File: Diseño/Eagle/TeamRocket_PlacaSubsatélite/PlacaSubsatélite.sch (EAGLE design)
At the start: 8 parts, among them IC2 7806DT

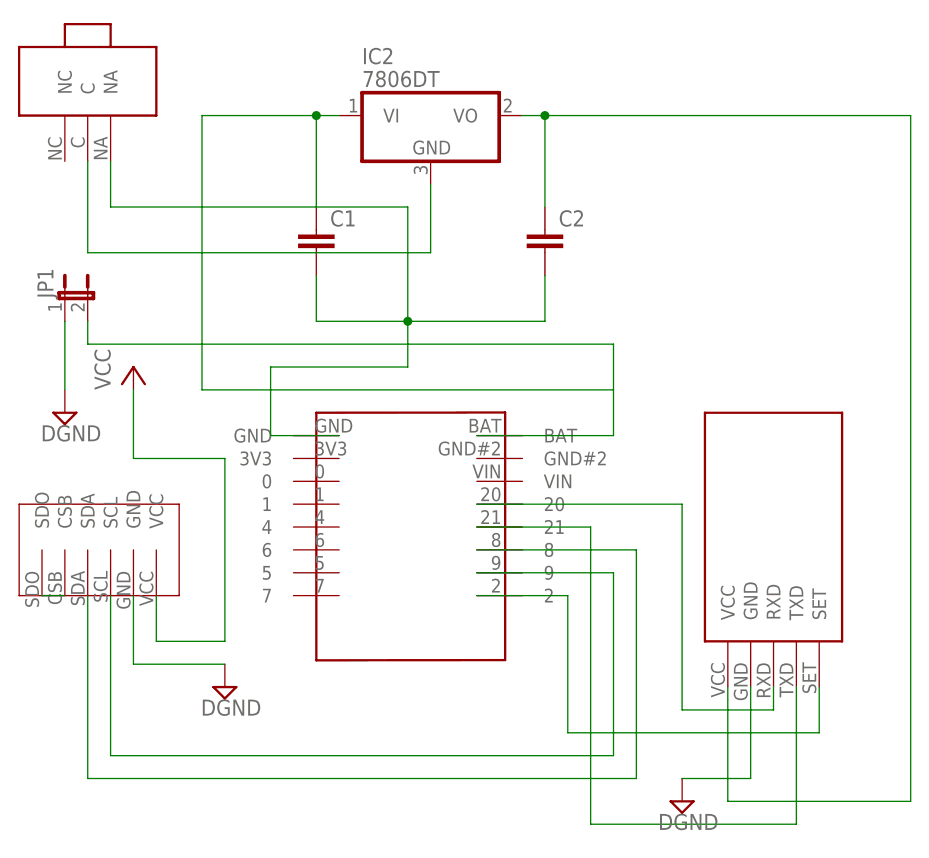
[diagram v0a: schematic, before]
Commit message: Update
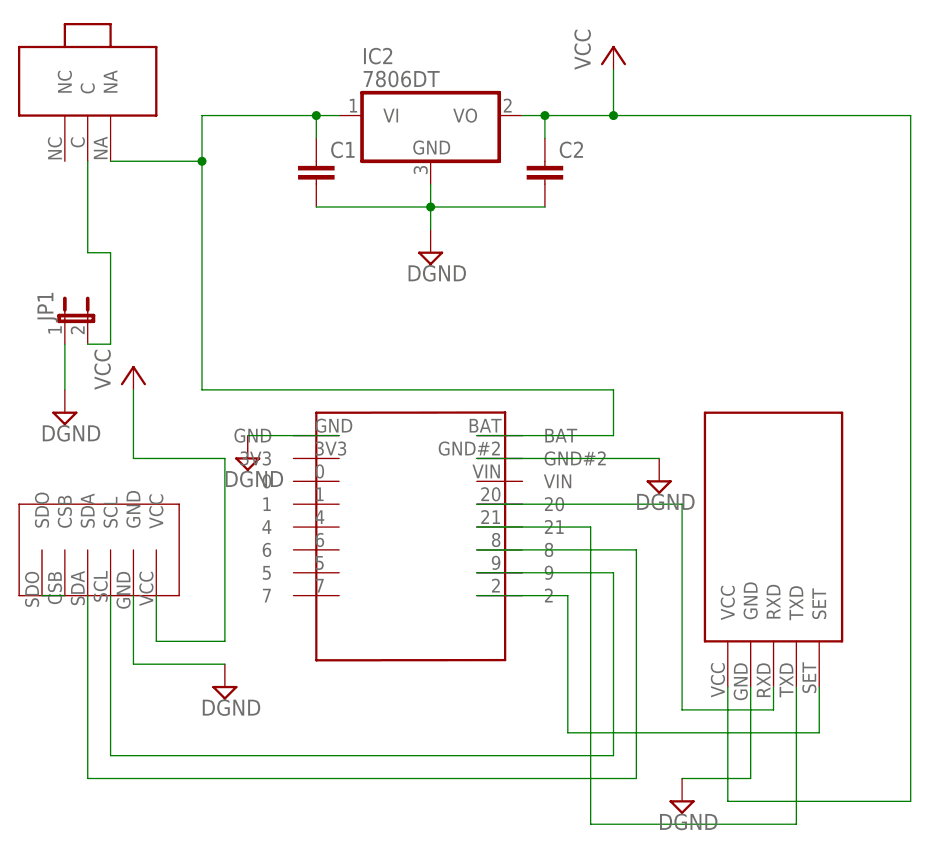
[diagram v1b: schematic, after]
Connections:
- removed net N$10: C2.1, IC2.VO, U$2.VCC
- removed net N$12: C1.2, C2.2, U$3.GND, U$4.NA
- net DGND: now also C1.2, C2.2, IC2.GND, U$3.GND, U$3.GND#2
- net N$1: now also U$4.NA; no longer JP1.2
- net N$2: now also JP1.2; no longer IC2.GND
- net VCC: now also C2.1, IC2.VO, U$2.VCC
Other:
- moved on the sheet: C1, C2, JP1
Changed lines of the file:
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@@
 <part name="SUPPLY3" library="supply2" library_urn="urn:adsk.eagle:library:372" deviceset="DGND" device=""/>
 <part name="U$4" library="switch" deviceset="SWITCH" device=""/>
+<part name="P+2" library="supply1" library_urn="urn:adsk.eagle:library:371" deviceset="VCC" device=""/>
+<part name="SUPPLY4" library="supply2" library_urn="urn:adsk.eagle:library:372" deviceset="DGND" device=""/>
+<part name="SUPPLY5" library="supply2" library_urn="urn:adsk.eagle:library:372" deviceset="DGND" device=""/>
+<part name="SUPPLY6" library="supply2" library_urn="urn:adsk.eagle:library:372" deviceset="DGND" device=""/>
 </parts>
 <sheets>
@@
 <attribute name="VALUE" x="-2.54" y="48.895" size="1.778" layer="96"/>
 </instance>
-<instance part="C1" gate="G$1" x="-7.62" y="33.02" smashed="yes">
-<attribute name="NAME" x="-6.096" y="33.401" size="1.778" layer="95"/>
-<attribute name="VALUE" x="-6.096" y="28.321" size="1.778" layer="96"/>
-</instance>
-<instance part="C2" gate="G$1" x="17.78" y="33.02" smashed="yes">
-<attribute name="NAME" x="19.304" y="33.401" size="1.778" layer="95"/>
-<attribute name="VALUE" x="19.304" y="28.321" size="1.778" layer="96"/>
+<instance part="C1" gate="G$1" x="-7.62" y="40.64" smashed="yes">
+<attribute name="NAME" x="-6.096" y="41.021" size="1.778" layer="95"/>
+<attribute name="VALUE" x="-6.096" y="35.941" size="1.778" layer="96"/>
+</instance>
+<instance part="C2" gate="G$1" x="17.78" y="40.64" smashed="yes">
+<attribute name="NAME" x="19.304" y="41.021" size="1.778" layer="95"/>
+<attribute name="VALUE" x="19.304" y="35.941" size="1.778" layer="96"/>
 </instance>
 <instance part="SUPPLY1" gate="G$1" x="-17.78" y="-17.78" smashed="yes">
@@
 <attribute name="VALUE" x="-30.48" y="15.24" size="1.778" layer="96" rot="R90"/>
 </instance>
-<instance part="JP1" gate="A" x="-35.56" y="25.4" smashed="yes">
-<attribute name="NAME" x="-36.83" y="25.4" size="1.778" layer="95" rot="R90"/>
-<attribute name="VALUE" x="-29.845" y="25.4" size="1.778" layer="96" rot="R90"/>
+<instance part="JP1" gate="A" x="-35.56" y="22.86" smashed="yes">
+<attribute name="NAME" x="-36.83" y="22.86" size="1.778" layer="95" rot="R90"/>
+<attribute name="VALUE" x="-29.845" y="22.86" size="1.778" layer="96" rot="R90"/>
 </instance>
 <instance part="SUPPLY3" gate="G$1" x="-35.56" y="12.7" smashed="yes">
@@
 </instance>
 <instance part="U$4" gate="G$1" x="-22.86" y="48.26" smashed="yes"/>
+<instance part="P+2" gate="VCC" x="25.4" y="53.34" smashed="yes">
+<attribute name="VALUE" x="22.86" y="50.8" size="1.778" layer="96" rot="R90"/>
+</instance>
+<instance part="SUPPLY4" gate="G$1" x="5.08" y="30.48" smashed="yes">
+<attribute name="VALUE" x="2.413" y="27.305" size="1.778" layer="96"/>
+</instance>
+<instance part="SUPPLY5" gate="G$1" x="-15.24" y="7.62" smashed="yes">
+<attribute name="VALUE" x="-17.907" y="4.445" size="1.778" layer="96"/>
+</instance>
+<instance part="SUPPLY6" gate="G$1" x="30.48" y="5.08" smashed="yes">
+<attribute name="VALUE" x="27.813" y="1.905" size="1.778" layer="96"/>
+</instance>
 </instances>
 <busses>
@@
 <pinref part="C1" gate="G$1" pin="1"/>
 <pinref part="IC2" gate="A1" pin="VI"/>
-<wire x1="-7.62" y1="45.72" x2="-7.62" y2="35.56" width="0.1524" layer="91"/>
+<wire x1="-7.62" y1="45.72" x2="-7.62" y2="43.18" width="0.1524" layer="91"/>
 <wire x1="-5.08" y1="45.72" x2="-7.62" y2="45.72" width="0.1524" layer="91"/>
 <wire x1="-20.32" y1="45.72" x2="-7.62" y2="45.72" width="0.1524" layer="91"/>
-<wire x1="-20.32" y1="45.72" x2="-20.32" y2="15.24" width="0.1524" layer="91"/>
+<wire x1="-20.32" y1="45.72" x2="-20.32" y2="40.64" width="0.1524" layer="91"/>
+<wire x1="-20.32" y1="40.64" x2="-20.32" y2="15.24" width="0.1524" layer="91"/>
 <wire x1="-20.32" y1="15.24" x2="25.4" y2="15.24" width="0.1524" layer="91"/>
 <pinref part="U$3" gate="G$1" pin="BAT"/>
 <wire x1="25.4" y1="15.24" x2="25.4" y2="10.16" width="0.1524" layer="91"/>
 <wire x1="25.4" y1="10.16" x2="10.2108" y2="10.16" width="0.1524" layer="91"/>
-<pinref part="JP1" gate="A" pin="2"/>
-<wire x1="-33.02" y1="22.86" x2="-33.02" y2="20.32" width="0.1524" layer="91"/>
-<wire x1="-33.02" y1="20.32" x2="25.4" y2="20.32" width="0.1524" layer="91"/>
-<wire x1="25.4" y1="20.32" x2="25.4" y2="15.24" width="0.1524" layer="91"/>
+<pinref part="U$4" gate="G$1" pin="NA"/>
+<wire x1="-30.48" y1="40.64" x2="-20.32" y2="40.64" width="0.1524" layer="91"/>
+<junction x="-20.32" y="40.64"/>
 </segment>
 </net>
@@
 </segment>
 </net>
-<net name="N$12" class="0">
-<segment>
-<pinref part="C1" gate="G$1" pin="2"/>
-<wire x1="2.54" y1="22.86" x2="-7.62" y2="22.86" width="0.1524" layer="91"/>
-<wire x1="-7.62" y1="27.94" x2="-7.62" y2="22.86" width="0.1524" layer="91"/>
-<pinref part="U$4" gate="G$1" pin="NA"/>
-<wire x1="-30.48" y1="40.64" x2="-30.48" y2="35.56" width="0.1524" layer="91"/>
-<wire x1="-30.48" y1="35.56" x2="2.54" y2="35.56" width="0.1524" layer="91"/>
-<wire x1="2.54" y1="35.56" x2="2.54" y2="22.86" width="0.1524" layer="91"/>
-<pinref part="U$3" gate="G$1" pin="GND"/>
-<wire x1="-5.08" y1="10.16" x2="-12.7" y2="10.16" width="0.1524" layer="91"/>
-<wire x1="2.54" y1="22.86" x2="2.54" y2="17.78" width="0.1524" layer="91"/>
-<wire x1="2.54" y1="17.78" x2="-12.7" y2="17.78" width="0.1524" layer="91"/>
-<wire x1="-12.7" y1="17.78" x2="-12.7" y2="10.16" width="0.1524" layer="91"/>
-<junction x="2.54" y="22.86"/>
-<pinref part="C2" gate="G$1" pin="2"/>
-<wire x1="17.78" y1="27.94" x2="17.78" y2="22.86" width="0.1524" layer="91"/>
-<wire x1="2.54" y1="22.86" x2="17.78" y2="22.86" width="0.1524" layer="91"/>
-</segment>
-</net>
-<net name="N$10" class="0">
-<segment>
-<pinref part="IC2" gate="A1" pin="VO"/>
-<wire x1="15.24" y1="45.72" x2="17.78" y2="45.72" width="0.1524" layer="91"/>
-<pinref part="C2" gate="G$1" pin="1"/>
-<wire x1="17.78" y1="45.72" x2="17.78" y2="35.56" width="0.1524" layer="91"/>
-<wire x1="17.78" y1="45.72" x2="58.42" y2="45.72" width="0.1524" layer="91"/>
-<pinref part="U$2" gate="G$1" pin="VCC"/>
-<wire x1="58.42" y1="-30.48" x2="38.1" y2="-30.48" width="0.1524" layer="91"/>
-<wire x1="38.1" y1="-30.48" x2="38.1" y2="-17.78" width="0.1524" layer="91"/>
-<wire x1="58.42" y1="45.72" x2="58.42" y2="-30.48" width="0.1524" layer="91"/>
-<junction x="17.78" y="45.72"/>
-</segment>
-</net>
 <net name="N$11" class="0">
 <segment>
@@
 <segment>
 <pinref part="JP1" gate="A" pin="1"/>
-<wire x1="-35.56" y1="22.86" x2="-35.56" y2="15.24" width="0.1524" layer="91"/>
+<wire x1="-35.56" y1="20.32" x2="-35.56" y2="15.24" width="0.1524" layer="91"/>
 <pinref part="SUPPLY3" gate="G$1" pin="DGND"/>
+</segment>
+<segment>
+<pinref part="C1" gate="G$1" pin="2"/>
+<pinref part="SUPPLY4" gate="G$1" pin="DGND"/>
+<wire x1="-7.62" y1="35.56" x2="5.08" y2="35.56" width="0.1524" layer="91"/>
+<wire x1="5.08" y1="35.56" x2="5.08" y2="33.02" width="0.1524" layer="91"/>
+<pinref part="C2" gate="G$1" pin="2"/>
+<wire x1="17.78" y1="35.56" x2="5.08" y2="35.56" width="0.1524" layer="91"/>
+<junction x="5.08" y="35.56"/>
+<pinref part="IC2" gate="A1" pin="GND"/>
+<wire x1="5.08" y1="38.1" x2="5.08" y2="35.56" width="0.1524" layer="91"/>
+</segment>
+<segment>
+<pinref part="U$3" gate="G$1" pin="GND"/>
+<wire x1="-5.08" y1="10.16" x2="-15.24" y2="10.16" width="0.1524" layer="91"/>
+<pinref part="SUPPLY5" gate="G$1" pin="DGND"/>
+</segment>
+<segment>
+<pinref part="U$3" gate="G$1" pin="GND#2"/>
+<pinref part="SUPPLY6" gate="G$1" pin="DGND"/>
+<wire x1="10.2108" y1="7.62" x2="30.48" y2="7.62" width="0.1524" layer="91"/>
 </segment>
 </net>
@@
 <wire x1="-27.94" y1="7.62" x2="-27.94" y2="15.24" width="0.1524" layer="91"/>
 </segment>
+<segment>
+<pinref part="IC2" gate="A1" pin="VO"/>
+<wire x1="15.24" y1="45.72" x2="17.78" y2="45.72" width="0.1524" layer="91"/>
+<pinref part="C2" gate="G$1" pin="1"/>
+<wire x1="17.78" y1="45.72" x2="17.78" y2="43.18" width="0.1524" layer="91"/>
+<wire x1="17.78" y1="45.72" x2="25.4" y2="45.72" width="0.1524" layer="91"/>
+<pinref part="U$2" gate="G$1" pin="VCC"/>
+<wire x1="25.4" y1="45.72" x2="58.42" y2="45.72" width="0.1524" layer="91"/>
+<wire x1="58.42" y1="-30.48" x2="38.1" y2="-30.48" width="0.1524" layer="91"/>
+<wire x1="38.1" y1="-30.48" x2="38.1" y2="-17.78" width="0.1524" layer="91"/>
+<wire x1="58.42" y1="45.72" x2="58.42" y2="-30.48" width="0.1524" layer="91"/>
+<junction x="17.78" y="45.72"/>
+<pinref part="P+2" gate="VCC" pin="VCC"/>
+<wire x1="25.4" y1="45.72" x2="25.4" y2="50.8" width="0.1524" layer="91"/>
+<junction x="25.4" y="45.72"/>
+</segment>
 </net>
 <net name="N$2" class="0">
 <segment>
-<pinref part="IC2" gate="A1" pin="GND"/>
-<wire x1="5.08" y1="38.1" x2="5.08" y2="30.48" width="0.1524" layer="91"/>
+<pinref part="JP1" gate="A" pin="2"/>
+<wire x1="-33.02" y1="20.32" x2="-30.48" y2="20.32" width="0.1524" layer="91"/>
+<wire x1="-30.48" y1="20.32" x2="-30.48" y2="30.48" width="0.1524" layer="91"/>
+<wire x1="-30.48" y1="30.48" x2="-33.02" y2="30.48" width="0.1524" layer="91"/>
 <pinref part="U$4" gate="G$1" pin="C"/>
-<wire x1="5.08" y1="30.48" x2="-33.02" y2="30.48" width="0.1524" layer="91"/>
 <wire x1="-33.02" y1="30.48" x2="-33.02" y2="40.64" width="0.1524" layer="91"/>
 </segment>
